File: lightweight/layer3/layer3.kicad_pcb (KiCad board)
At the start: 2 copper layers, 189.7 x 105 mm, 62 parts, among them J1 SH1.0 5P, J10 SH1.0 2P, J11 SH1.0 5P, J2 SH1.0 5P, J3 SH1.0 5P, J6 SH1.0 Female, J8 COMPASS, SW1 SW_SPDT, SW5 SW_Push, U1 TEENSY 4.0, U2 MOUDLE-SEEEDUINO-XIAO-ESP32C3, U3 BNO085, U5 74LVC2G04, U6 74LVC2G04, U7 STM32F103C8T6, Y1 Crystal

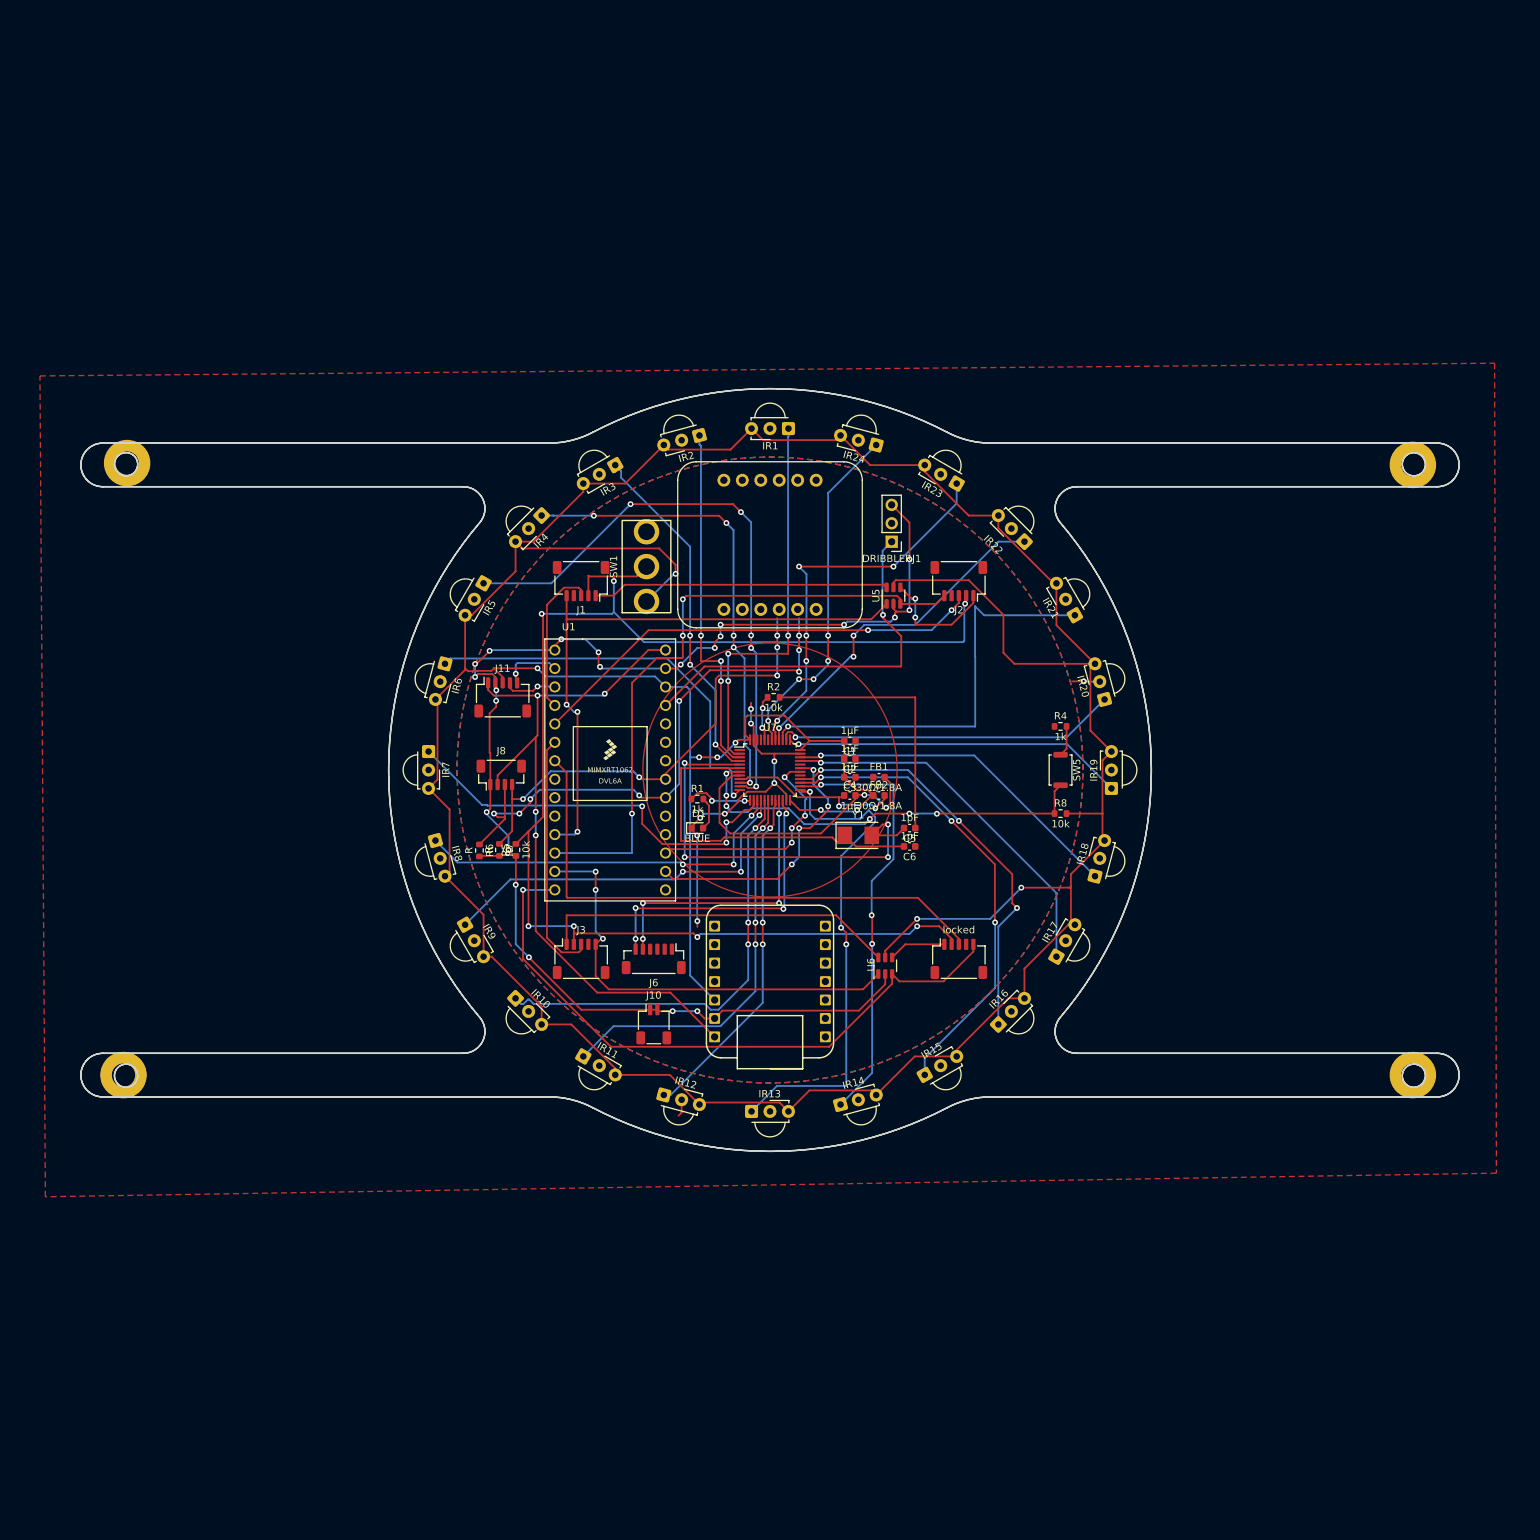
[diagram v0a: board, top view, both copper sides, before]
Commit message: update lw pcbs
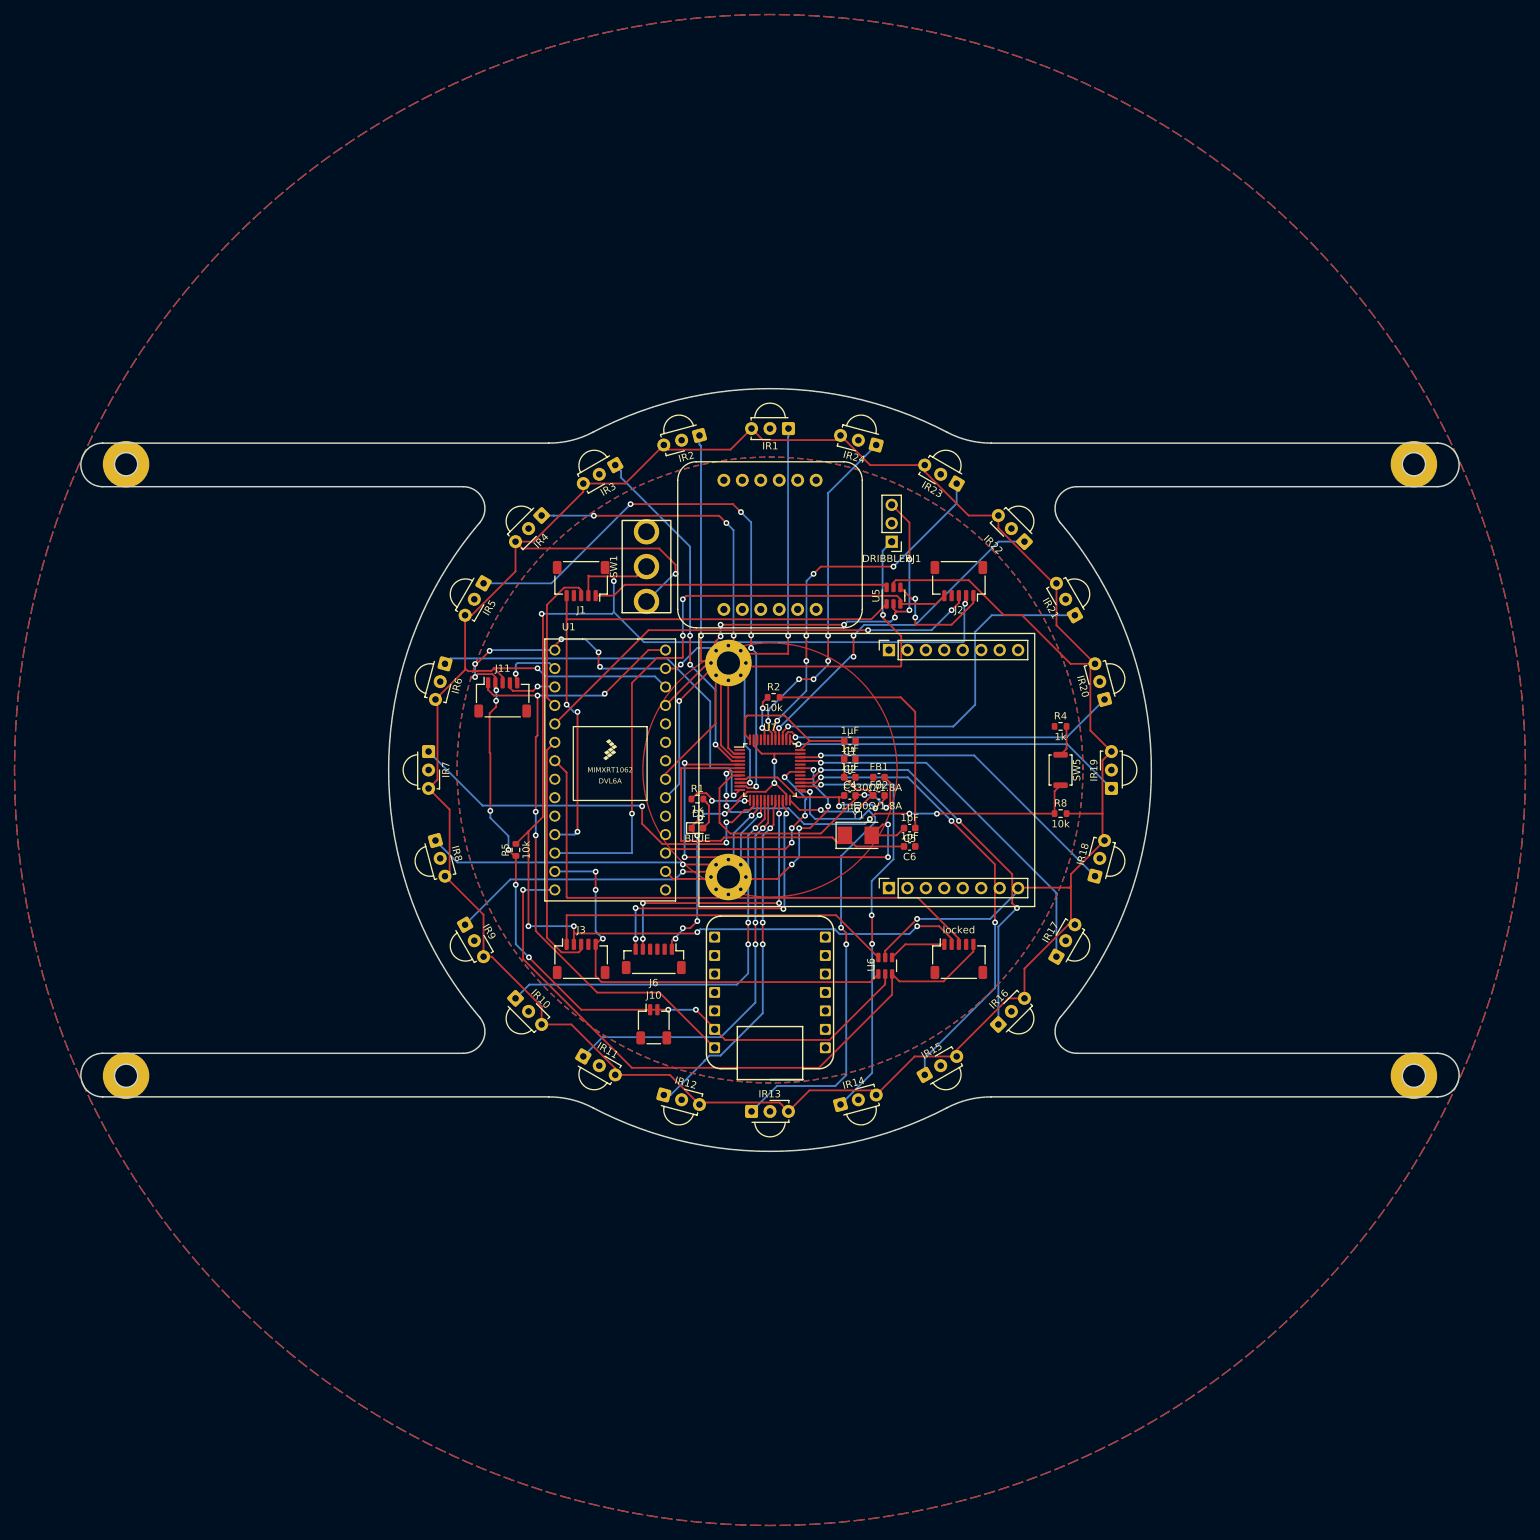
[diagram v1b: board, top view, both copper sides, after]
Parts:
- removed J8: COMPASS, Connector_JST:JST_SH_BM04B-SRSS-TB_1x04-1MP_P1.00mm_Vertical
- removed R6, R7: R, Resistor_SMD:R_0603_1608Metric
- added J5: Conn_01x16_Socket, footprints:openmv, F.Cu at (98.8, 105.0)
- moved U2 1.50 mm to (105.0, 135.6)
- moved H3 0.37 mm to (16.4, 147.1)
- moved H1 0.21 mm to (16.4, 62.9)
- moved H2 0.17 mm to (193.6, 62.9)
- moved H4 0.17 mm to (193.6, 147.1)
- renumbered U3 to U4
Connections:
- U4 pad JP1_1: (no net) -> +3V3
- U4 pad JP1_2: (no net) -> unconnected-(U4-3VO-PadJP1_2)
- U4 pad JP1_3: (no net) -> GND
- U4 pad JP1_4: (no net) -> /IMUSCL
- U4 pad JP1_5: (no net) -> /IMUSDA
- U4 pad JP1_6: (no net) -> unconnected-(U4-~{INT}-PadJP1_6)
- U4 pad JP2_1: (no net) -> unconnected-(U4-BT-PadJP2_1)
- U4 pad JP2_2: (no net) -> unconnected-(U4-P0-PadJP2_2)
- U4 pad JP2_3: (no net) -> unconnected-(U4-P1-PadJP2_3)
- U4 pad JP2_4: (no net) -> unconnected-(U4-~{RST}-PadJP2_4)
- U4 pad JP2_5: (no net) -> unconnected-(U4-DI-PadJP2_5)
- U4 pad JP2_6: (no net) -> unconnected-(U4-CS-PadJP2_6)
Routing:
- net +3V3: track 553.1 -> 493.2 mm, vias 9 -> 5
- net /IMUSDA: track 76.9 -> 20.1 mm, vias 8 -> 1
- net /IMUSCL: track 65.3 -> 17.3 mm, vias 5 -> 0
- net +5V: track 100.2 -> 92.1 mm
- net GND: track 91.1 -> 84.1 mm, vias 9 -> 8
- net /ir/IR21: track 58.7 -> 53.8 mm
- net /M4INA: track 88.9 -> 92.2 mm
- net Net-(R6-Pad2): track 2.78 -> 0.00 mm
- net /ir/IR2: track 48.8 -> 46.0 mm, vias 3 -> 1
- net /ir/IR23: track 54.4 -> 51.8 mm
- net /ir/IR10: track 60.6 -> 58.2 mm
- net GNDD: track 189.4 -> 190.8 mm, vias 22 -> 21
- net /ir/IR1: track 55.2 -> 54.2 mm, vias 3 -> 1
- net /DRIBBLERPWM: track 54.4 -> 53.4 mm
- net /ir/IR3: track 49.4 -> 48.5 mm
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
